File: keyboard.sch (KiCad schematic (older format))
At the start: 18 parts, among them IC1 ATMEGA32U4, J1 USBMINI_B05, P1 ISP, P2 GPIO Port, X1 CRYSTAL

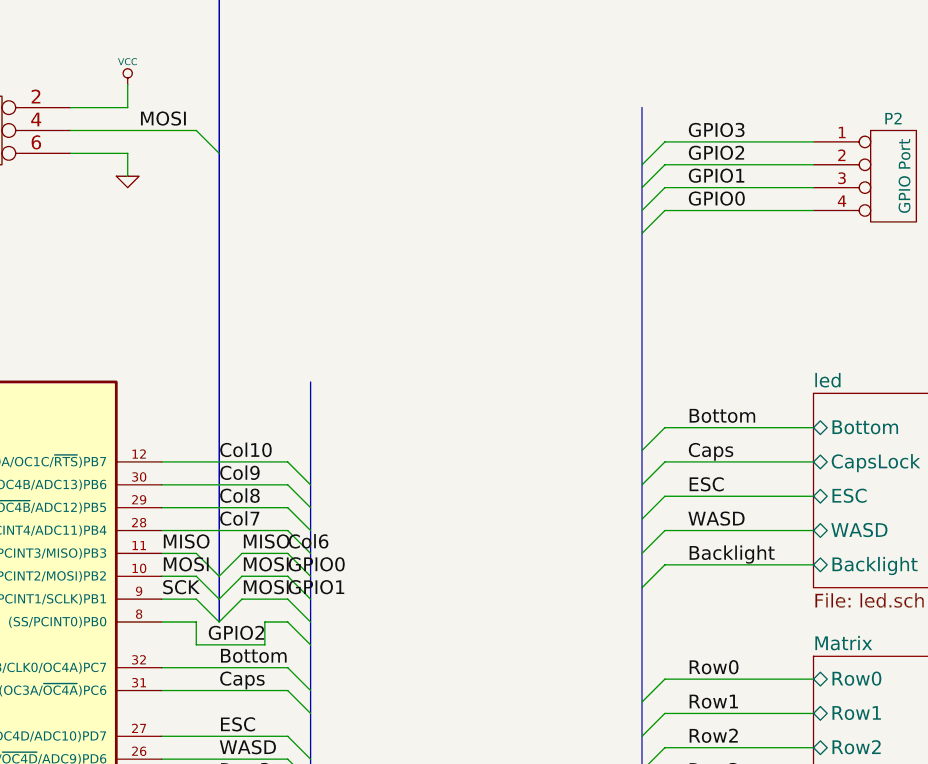
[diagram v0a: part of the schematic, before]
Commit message: a lot of changes
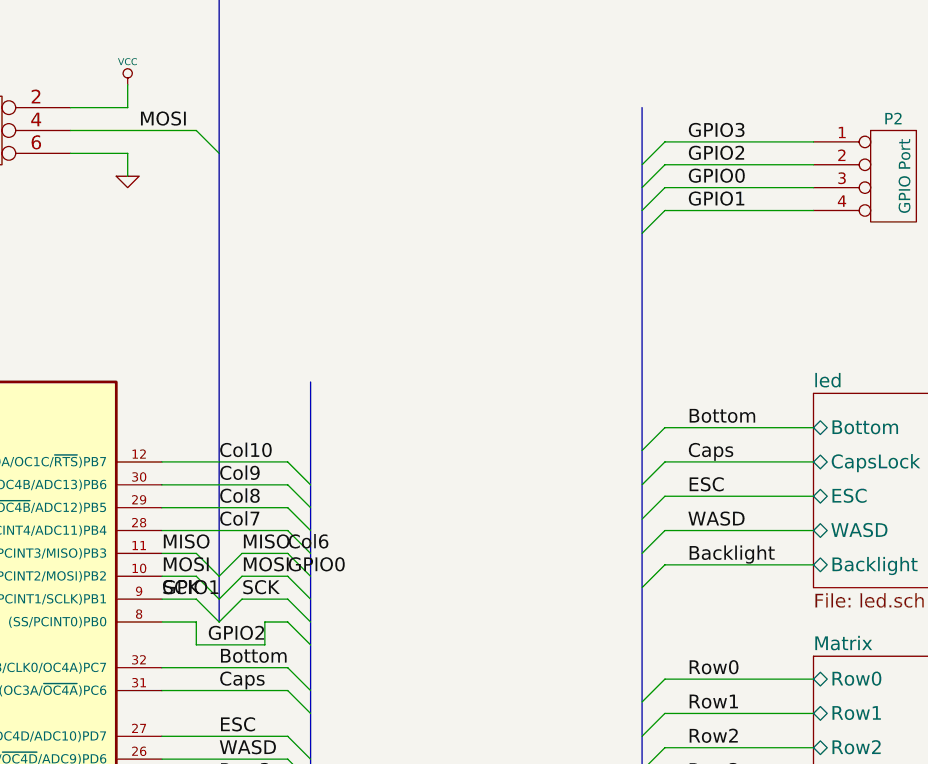
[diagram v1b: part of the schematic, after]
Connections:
- net GPIO0: no longer P2.4 (P4)
- net SCK renamed GPIO1
- net GPIO1: now also P2.4 (P4)
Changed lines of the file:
@@
 MOSI
 Text Label 6400 3500 0    60   ~ 0
-MOSI
+SCK
 Text Label 6600 3300 0    60   ~ 0
 Col6
 Text Label 6600 3400 0    60   ~ 0
 GPIO0
-Text Label 6600 3500 0    60   ~ 0
+Text Label 6050 3500 0    60   ~ 0
 GPIO1
 Text Label 6250 3700 0    60   ~ 0
@@
 Text Label 8350 1600 0    60   ~ 0
 GPIO2
+Text Label 8350 1800 0    60   ~ 0
+GPIO1
 Text Label 8350 1700 0    60   ~ 0
-GPIO1
-Text Label 8350 1800 0    60   ~ 0
 GPIO0
 $Comp
